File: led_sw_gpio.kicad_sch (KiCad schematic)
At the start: 33 parts, among them Q6 2N7002, SW3 up, SW4 down, SW5 left, SW6 rigth, SW7 up, SW8 down

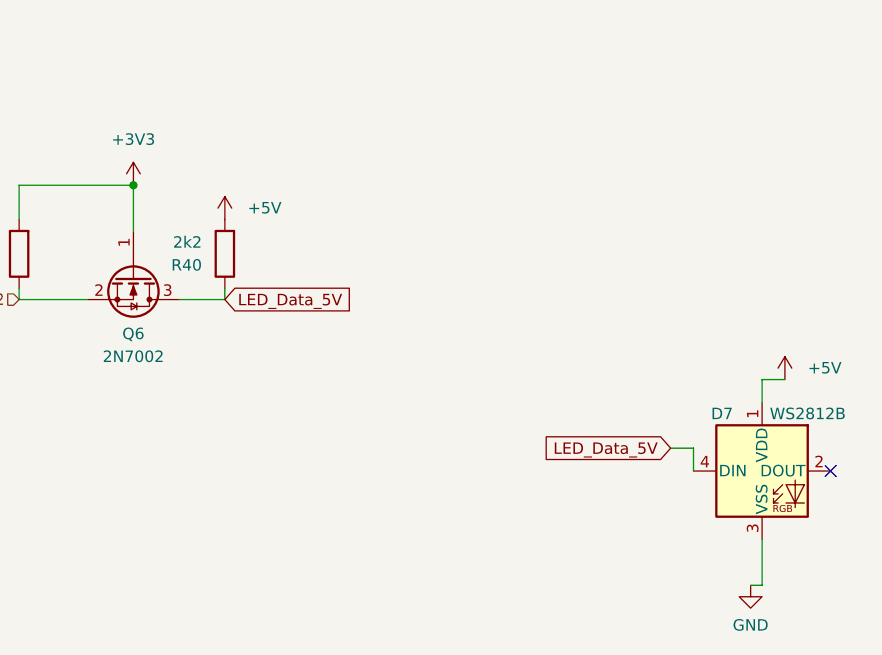
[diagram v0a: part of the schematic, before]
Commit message: Update schematics, PCB, and project files
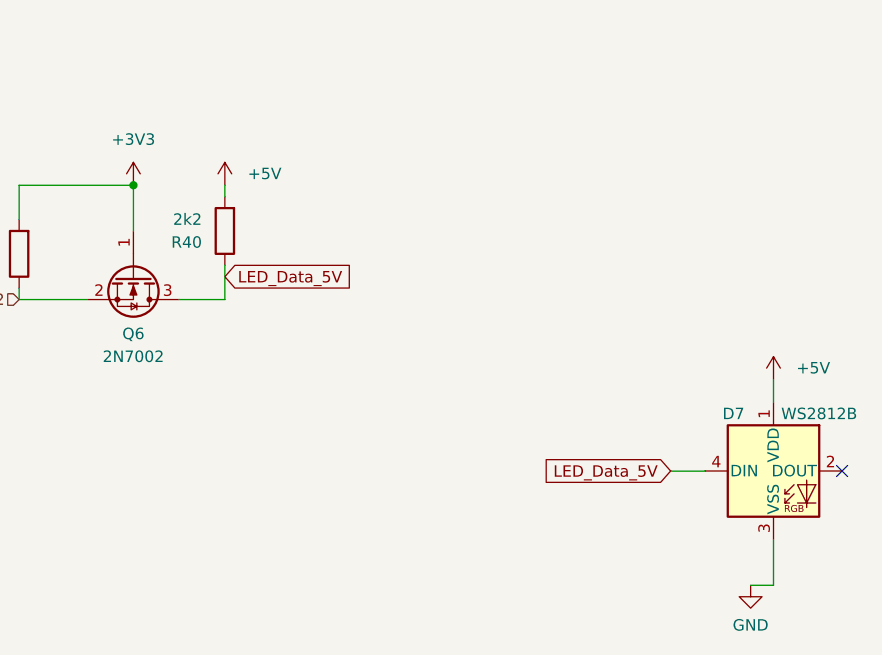
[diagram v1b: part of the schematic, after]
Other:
- moved on the sheet: D7, R40
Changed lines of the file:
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@@
 	)
 	(no_connect
-		(at 374.65 220.98)
+		(at 375.92 220.98)
 	)
 	(wire
@@
 	(wire
 		(pts
-			(xy 356.87 218.44) (xy 359.41 218.44)
+			(xy 356.87 220.98) (xy 360.68 220.98)
 		)
 		(stroke
@@
 	(wire
 		(pts
-			(xy 367.03 228.6) (xy 367.03 233.68)
+			(xy 368.3 228.6) (xy 368.3 233.68)
 		)
 		(stroke
@@
 	(wire
 		(pts
-			(xy 367.03 233.68) (xy 365.76 233.68)
+			(xy 368.3 233.68) (xy 365.76 233.68)
 		)
 		(stroke
@@
 	(wire
 		(pts
-			(xy 367.03 210.82) (xy 367.03 213.36)
+			(xy 368.3 210.82) (xy 368.3 213.36)
 		)
 		(stroke
@@
 	(wire
 		(pts
-			(xy 307.34 201.93) (xy 307.34 200.66)
-		)
-		(stroke
-			(width 0)
-			(type default)
-		)
-	)
-	(wire
-		(pts
-			(xy 359.41 218.44) (xy 359.41 220.98)
+			(xy 307.34 201.93) (xy 307.34 198.12)
 		)
 		(stroke
@@
 	(wire
 		(pts
-			(xy 367.03 210.82) (xy 369.57 210.82)
+			(xy 125.73 105.41) (xy 125.73 116.84)
 		)
 		(stroke
@@
 	(wire
 		(pts
-			(xy 125.73 105.41) (xy 125.73 116.84)
+			(xy 234.95 101.6) (xy 234.95 114.3)
 		)
 		(stroke
@@
 	(wire
 		(pts
-			(xy 234.95 101.6) (xy 234.95 114.3)
+			(xy 273.05 154.94) (xy 273.05 143.51)
 		)
 		(stroke
@@
 	(wire
 		(pts
-			(xy 273.05 154.94) (xy 273.05 143.51)
+			(xy 307.34 189.23) (xy 307.34 190.5)
 		)
 		(stroke
@@
 	(global_label "LED_Data_5V"
 		(shape input)
-		(at 307.34 201.93 0)
+		(at 307.34 199.39 0)
 		(fields_autoplaced yes)
 		(effects
@@
 		)
 		(property "Intersheetrefs" "${INTERSHEET_REFS}"
-			(at 322.2993 201.93 0)
+			(at 322.2993 199.39 0)
 			(hide yes)
 			(show_name no)
@@
 	(global_label "LED_Data_5V"
 		(shape input)
-		(at 356.87 218.44 180)
+		(at 356.87 220.98 180)
 		(fields_autoplaced yes)
 		(effects
@@
 		)
 		(property "Intersheetrefs" "${INTERSHEET_REFS}"
-			(at 341.9901 218.44 0)
+			(at 341.9901 220.98 0)
 			(hide yes)
 			(show_name no)
@@
 	(symbol
 		(lib_id "power:+5V")
-		(at 369.57 210.82 0)
+		(at 368.3 210.82 0)
 		(unit 1)
 		(body_style 1)
@@
 		(fields_autoplaced yes)
 		(property "Reference" "#PWR065"
-			(at 369.57 214.63 0)
+			(at 368.3 214.63 0)
 			(hide yes)
 			(show_name no)
@@
 		)
 		(property "Value" "+5V"
-			(at 372.11 209.5499 0)
+			(at 370.84 209.5499 0)
 			(show_name no)
 			(do_not_autoplace no)
@@
 		)
 		(property "Footprint" ""
-			(at 369.57 210.82 0)
+			(at 368.3 210.82 0)
 			(hide yes)
 			(show_name no)
@@
 		)
 		(property "Datasheet" ""
-			(at 369.57 210.82 0)
+			(at 368.3 210.82 0)
 			(hide yes)
 			(show_name no)
@@
 		)
 		(property "Description" ""
-			(at 369.57 210.82 0)
+			(at 368.3 210.82 0)
 			(show_name no)
 			(do_not_autoplace no)
@@
 	(symbol
 		(lib_id "LED:WS2812B")
-		(at 367.03 220.98 0)
+		(at 368.3 220.98 0)
 		(unit 1)
 		(body_style 1)
@@
 		(dnp no)
 		(property "Reference" "D7"
-			(at 362.585 214.63 0)
+			(at 363.855 214.63 0)
 			(show_name no)
 			(do_not_autoplace no)
@@
 		)
 		(property "Value" "WS2812B"
-			(at 372.11 214.63 0)
+			(at 373.38 214.63 0)
 			(show_name no)
 			(do_not_autoplace no)
@@
 		)
 		(property "Footprint" "LED_SMD:LED_WS2812B_PLCC4_5.0x5.0mm_P3.2mm"
-			(at 368.3 228.6 0)
+			(at 369.57 228.6 0)
 			(hide yes)
 			(show_name no)
@@
 		)
 		(property "Datasheet" "https://cdn-shop.adafruit.com/datasheets/WS2812B.pdf"
-			(at 369.57 230.505 0)
+			(at 370.84 230.505 0)
 			(hide yes)
 			(show_name no)
@@
 		)
 		(property "Description" ""
-			(at 367.03 220.98 0)
+			(at 368.3 220.98 0)
 			(show_name no)
 			(do_not_autoplace no)
@@
 		)
 		(property "LCSC Part #" "C2761795"
-			(at 367.03 220.98 0)
+			(at 368.3 220.98 0)
 			(hide yes)
 			(show_name no)
@@
 	(symbol
 		(lib_id "power:+5V")
-		(at 307.34 193.04 0)
+		(at 307.34 189.23 0)
 		(unit 1)
 		(body_style 1)
@@
 		(fields_autoplaced yes)
 		(property "Reference" "#PWR063"
-			(at 307.34 196.85 0)
+			(at 307.34 193.04 0)
 			(hide yes)
 			(show_name no)
@@
 		)
 		(property "Value" "+5V"
-			(at 309.88 191.7699 0)
+			(at 309.88 187.9599 0)
 			(show_name no)
 			(do_not_autoplace no)
@@
 		)
 		(property "Footprint" ""
-			(at 307.34 193.04 0)
+			(at 307.34 189.23 0)
 			(hide yes)
 			(show_name no)
@@
 		)
 		(property "Datasheet" ""
-			(at 307.34 193.04 0)
+			(at 307.34 189.23 0)
 			(hide yes)
 			(show_name no)
@@
 		)
 		(property "Description" ""
-			(at 307.34 193.04 0)
+			(at 307.34 189.23 0)
 			(show_name no)
 			(do_not_autoplace no)
@@
 	(symbol
 		(lib_id "Device:R")
-		(at 307.34 196.85 180)
+		(at 307.34 194.31 180)
 		(unit 1)
 		(body_style 1)
@@
 		(fields_autoplaced yes)
 		(property "Reference" "R40"
-			(at 304.8 198.1201 0)
+			(at 304.8 195.5801 0)
 			(show_name no)
 			(do_not_autoplace no)
@@
 		)
 		(property "Value" "2k2"
-			(at 304.8 195.5801 0)
+			(at 304.8 193.0401 0)
 			(show_name no)
 			(do_not_autoplace no)
@@
 		)
 		(property "Footprint" "Resistor_SMD:R_0805_2012Metric"
-			(at 309.118 196.85 90)
+			(at 309.118 194.31 90)
 			(hide yes)
 			(show_name no)
@@
 		)
 		(property "Datasheet" ""
-			(at 307.34 196.85 0)
+			(at 307.34 194.31 0)
 			(hide yes)
 			(show_name no)
@@
 		)
 		(property "Description" ""
-			(at 307.34 196.85 0)
+			(at 307.34 194.31 0)
 			(show_name no)
 			(do_not_autoplace no)
